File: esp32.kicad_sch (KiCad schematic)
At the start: 45 parts, among them SW2 BOOT, U6 ESP32-S3R8, U7 W25Q128JVSIQ, Y1 40MHz

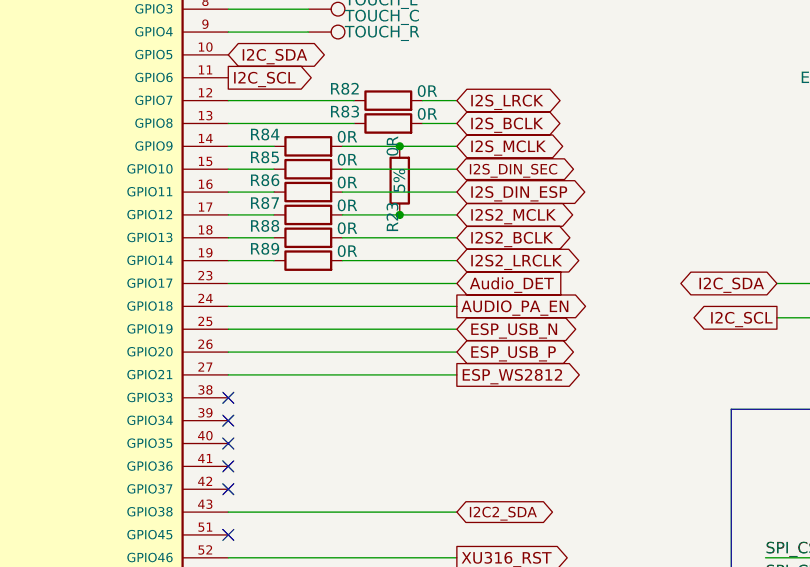
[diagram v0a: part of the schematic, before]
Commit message: mods after 1st batch testing
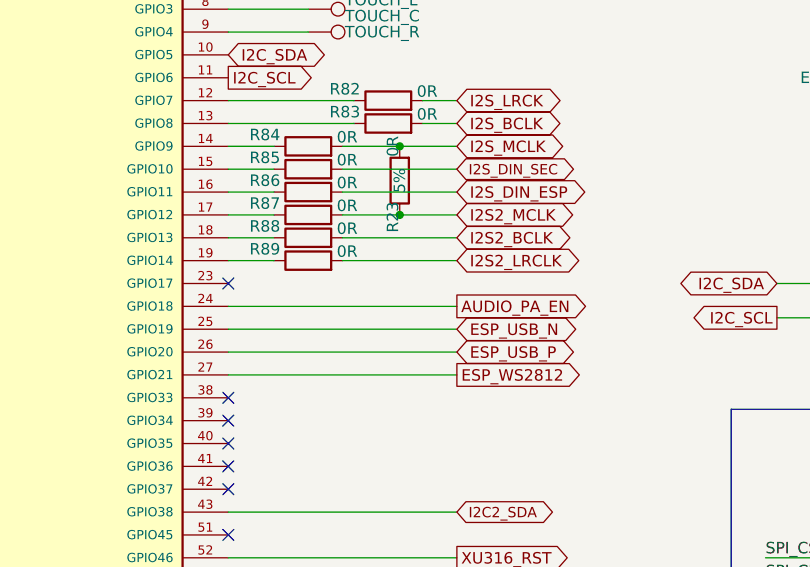
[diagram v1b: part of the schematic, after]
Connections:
- net Audio_DET: no longer names the net of U6.23 (GPIO17)
- no-connect marks 11 -> 12
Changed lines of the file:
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@@
+	)
+	(no_connect
+		(at 162.56 104.14)
 	)
 	(no_connect
@@
 		(pts
 			(xy 181.61 88.9) (xy 187.96 88.9)
-		)
-		(stroke
-			(width 0)
-			(type default)
-		)
-	)
-	(wire
-		(pts
-			(xy 187.96 104.14) (xy 162.56 104.14)
 		)
 		(stroke
@@
 			(effects
 				(font
-					(size 1.27 1.27)
-				)
-				(justify left)
-				(hide yes)
-			)
-		)
-	)
-	(global_label "Audio_DET"
-		(shape input)
-		(at 187.96 104.14 0)
-		(fields_autoplaced yes)
-		(effects
-			(font
-				(size 1.27 1.27)
-			)
-			(justify left)
-		)
-		(property "Intersheetrefs" "${INTERSHEET_REFS}"
-			(at 200.4398 104.14 0)
-			(effects
-				(font
